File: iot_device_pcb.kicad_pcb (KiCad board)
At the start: 4 copper layers, 75 x 73.9 mm, 74 parts, among them J1 B2B-PH-K-S_LF__SN_, J2 USB_C_Receptacle_USB2.0_16P, J3 Screw_Terminal_01x03, J4 Conn_01x04_Pin, J5 Conn_01x04_Pin, J6 Conn_01x07_Pin, K1 RAYEX-L90, Q1 BC817, Q2 BC817, Q3 BC817, U1 AMS1117-3.3, U2 MCP73871, U4 ESP32-S3-WROOM-1, U5 BME280, U6 MPU-6050

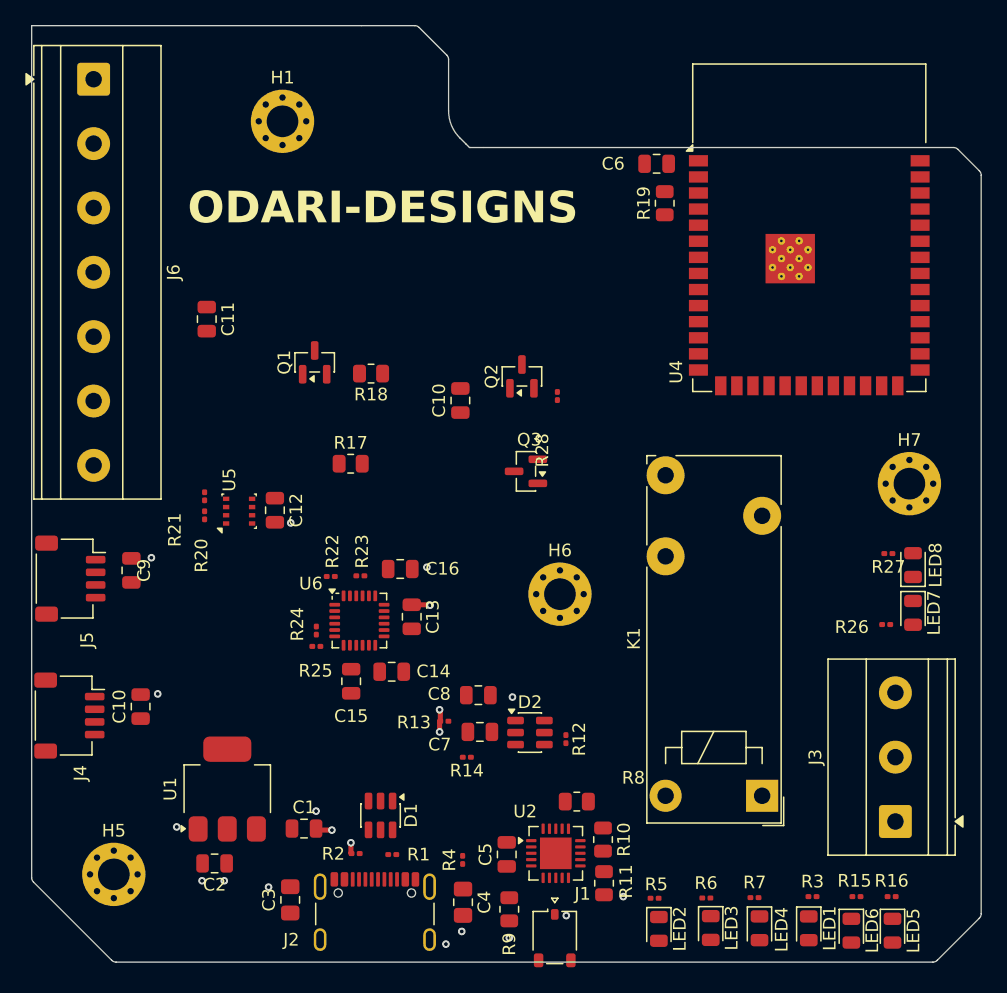
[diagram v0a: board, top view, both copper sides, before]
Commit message: chore(pcb): upgrade KiCad file format and plot settings
Update the PCB file to KiCad version 20260206 and generator 10.0.
Refactor plot parameters to include explicit tenting, covering,
plugging, and capping settings, and clean up legacy HPGL parameters.
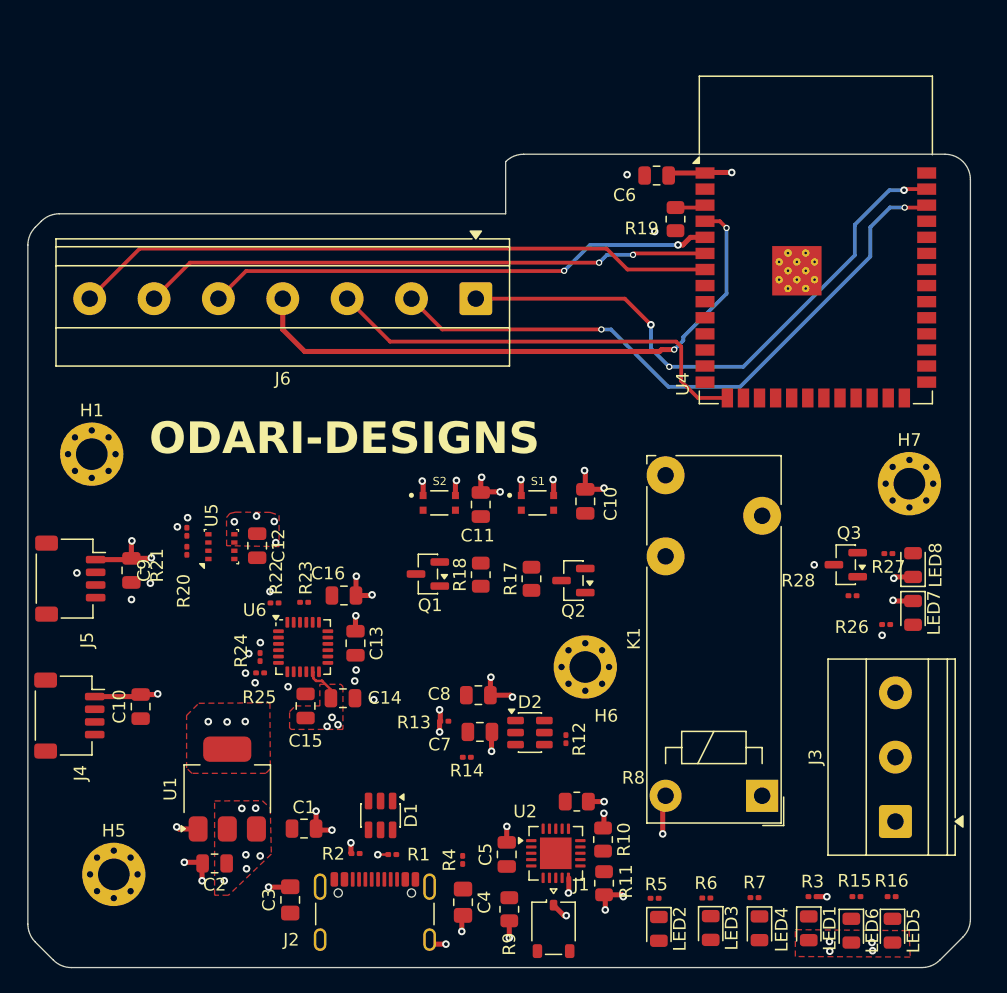
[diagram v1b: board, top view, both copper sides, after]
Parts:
- added S1: USLPT2819DT2TR, USLPT2819DT2TR:SW_USLPT2819DT2TR, F.Cu at (126.2, 120.4)
- added S2: USLPT2819DT2TR, USLPT2819DT2TR:SW_USLPT2819DT2TR, F.Cu at (118.5, 120.4)
- moved J6 34.8 mm to (121.4, 104.3), turned to 180 degrees
- moved H1 30.3 mm to (91.0, 116.6)
- moved R28 28.1 mm to (151.1, 127.8), turned to 180 degrees
- moved Q3 26.3 mm to (150.6, 125.3)
- moved C11 26.1 mm to (121.8, 120.5), turned to 90 degrees
- moved Q1 18.9 mm to (117.6, 126.0), turned to 180 degrees
- moved R18 18.1 mm to (121.8, 126.1), turned to 90 degrees
- moved R17 16.9 mm to (125.8, 126.4), turned to 90 degrees
- moved Q2 16.6 mm to (129.1, 126.5), turned to 180 degrees
- moved C10 12.7 mm to (130.0, 120.3)
- moved H6 6.09 mm to (130.0, 133.4)
- moved C13 4.91 mm to (111.9, 131.5)
- moved C16 4.91 mm to (111.0, 127.7)
- moved R23 4.91 mm to (107.8, 128.3)
- moved R24 4.91 mm to (104.3, 132.6)
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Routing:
- net GND: track 5.43 -> 71.3 mm, vias 20 -> 51
- net /Microcontroller-ESP32-S3-WROOM-1/GPIO7: track 0.00 -> 50.9 mm
- net /Microcontroller-ESP32-S3-WROOM-1/GPIO2: track 0.00 -> 50.9 mm, vias 0 -> 2
- net /Microcontroller-ESP32-S3-WROOM-1/GPIO4: track 0.00 -> 47.3 mm, vias 0 -> 2
- net /Microcontroller-ESP32-S3-WROOM-1/GPIO1: track 0.00 -> 46.3 mm, vias 0 -> 3
- net /Microcontroller-ESP32-S3-WROOM-1/GPIO6: track 0.00 -> 45.0 mm, vias 0 -> 2
- net /Microcontroller-ESP32-S3-WROOM-1/GPIO5: track 0.00 -> 40.4 mm, vias 0 -> 2
- net /Microcontroller-ESP32-S3-WROOM-1/GPIO3: track 0.00 -> 34.9 mm
- net /Microcontroller-ESP32-S3-WROOM-1/EN: track 0.00 -> 2.41 mm
- net +3.3V: vias 0 -> 29
- added copper zone on F.Cu, net +3.3V
- added copper zone on In2.Cu, net +3.3V
- added copper zone on F.Cu, net GND
- removed copper zone on In1.Cu, net GND
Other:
- board size 75 x 73.9 mm -> 74.4 x 64.2 mm
